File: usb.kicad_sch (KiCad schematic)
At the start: 22 parts, among them J1 USB4110, J2 USB_A, U4 MCIMX6Y2DVM09AB, U5 AP22615AWU-7

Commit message: Update fields
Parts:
- C33, C38, C39, C41: Manufacturer (none) -> Samsung Electro-Mechanics; MfgPartNo (none) -> CL21A106KPFNNNG; Vendor (none) -> Digi-Key; VendorPartNo (none) -> 1276-6456-1-ND
- C34, C35, C36: Manufacturer (none) -> TDK Corporation; MfgPartNo (none) -> CGB2A1X5R1E105K033BC; Vendor (none) -> Digi-Key; VendorPartNo (none) -> 445-13185-1-ND
- C37, C42: Manufacturer (none) -> Murata Electronics; MfgPartNo (none) -> GRM155R71H104KE14D; Vendor (none) -> Digi-Key; VendorPartNo (none) -> 490-10700-1-ND
- C40: Manufacturer (none) -> Samsung Electro-Mechanics; MfgPartNo (none) -> CL32A107MQVNNNE; Vendor (none) -> Digi-Key; VendorPartNo (none) -> 1276-1092-1-ND
- D2, D5: Manufacturer (none) -> Semtech Corporation; MfgPartNo (none) -> RCLRAMP0582B.TCT; Vendor (none) -> Digi-Key; VendorPartNo (none) -> RCLAMP0582B.TCTCT-ND
- D3, D4: Manufacturer (none) -> Semtech Corporation; MfgPartNo (none) -> UCLAMP0571P.TNT; Vendor (none) -> Digi-Key; VendorPartNo (none) -> UCLAMP0571P.TNTCT-ND
- J1: Manufacturer (none) -> GCT; MfgPartNo (none) -> USB4110-GF-A; Vendor (none) -> Digi-Key; VendorPartNo (none) -> 2073-USB4110-GF-A-1-ND
- J2: Manufacturer (none) -> Amphenol ICC (FCI); MfgPartNo (none) -> 87583-2010RLF; Vendor (none) -> Digi-Key; VendorPartNo (none) -> 609-5390-1-ND
- R10, R9: Manufacturer (none) -> YAGEO; MfgPartNo (none) -> RC0402FR-07510RL; Vendor (none) -> Digi-Key; VendorPartNo (none) -> 311-510LRCT-ND
- R11: Manufacturer (none) -> YAGEO; MfgPartNo (none) -> RC0402FR-07100KL; Vendor (none) -> Digi-Key; VendorPartNo (none) -> 311-100KLRCT-ND
- R12: Manufacturer (none) -> YAGEO; MfgPartNo (none) -> RC0402FR-136K8L; Vendor (none) -> Digi-Key; VendorPartNo (none) -> 13-RC0402FR-136K8LCT-ND
- U5: Manufacturer (none) -> Diodes Incorporated; MfgPartNo (none) -> AP22615AWU-7; Vendor (none) -> Digi-Key; VendorPartNo (none) -> AP22615AWU-7DICT-ND

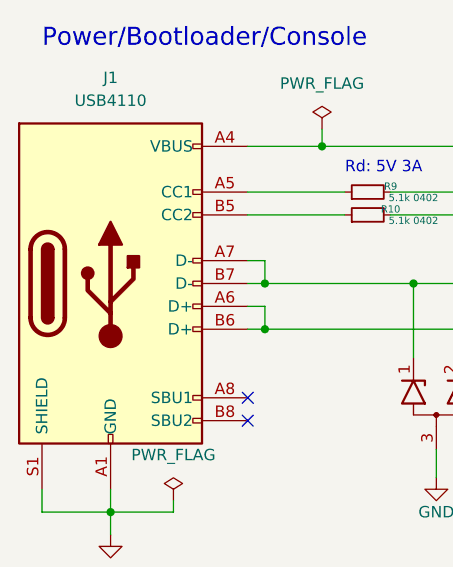
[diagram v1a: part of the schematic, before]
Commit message: KiCad 7
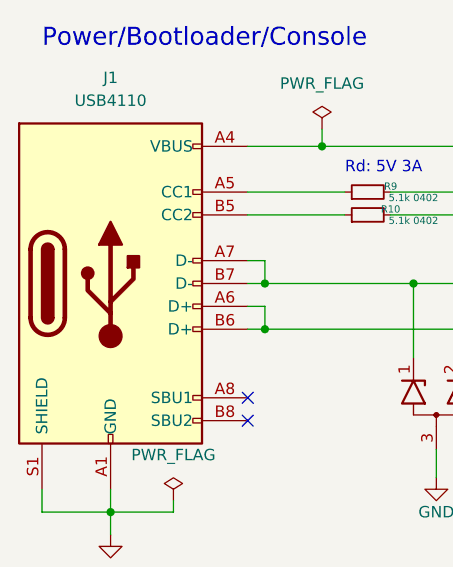
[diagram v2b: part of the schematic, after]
